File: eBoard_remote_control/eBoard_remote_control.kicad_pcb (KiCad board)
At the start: 2 copper layers, 34 x 99.9 mm, 57 parts, among them J1 SWDIO_conn, J2 105450-0101, U1 MDBT42, U2 AP2112(3.3V), U3 MCP73831T-2ACI/OT, U4 CP2104, U5 AH49ENTR-G1, U6 AH49ENTR-G1, U7 AH49ENTR-G1, U8 SSD1306, X1 JSTPH, X2 JSTPH, X4 32.768

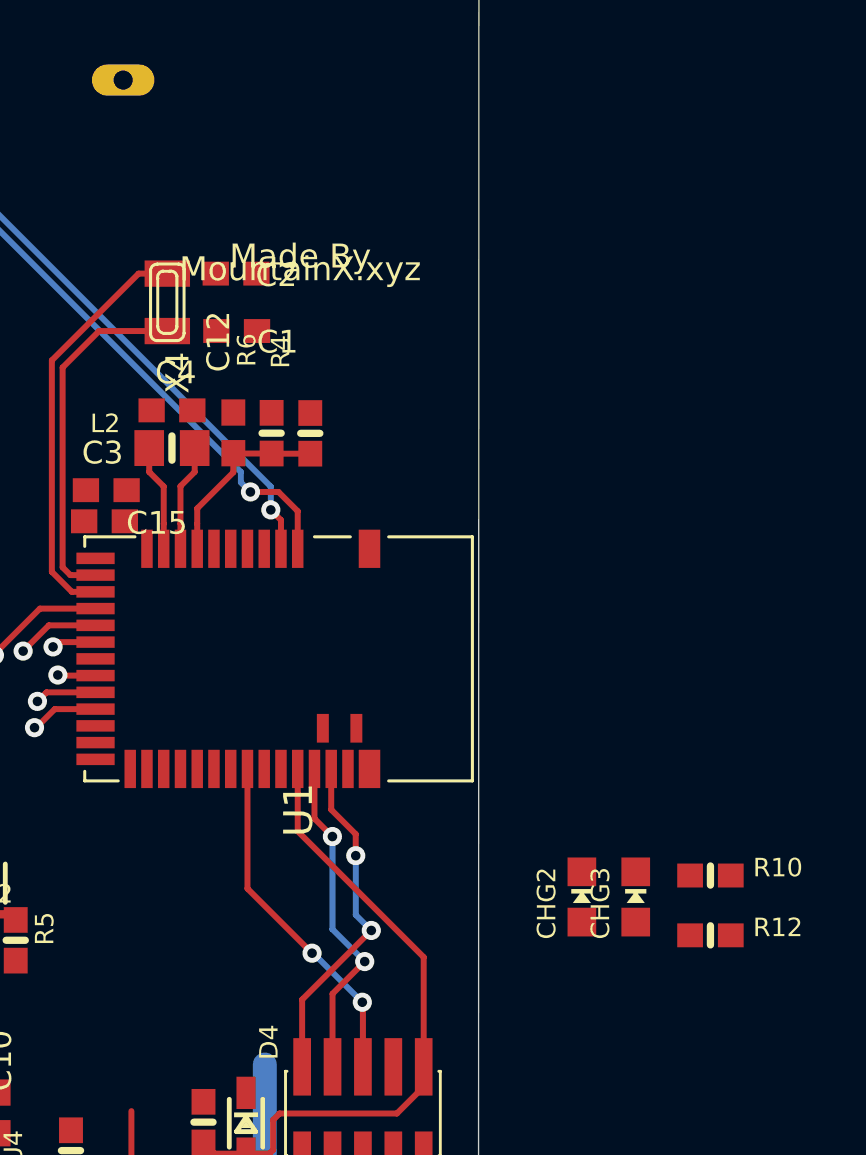
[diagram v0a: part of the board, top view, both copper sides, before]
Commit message: updated 3d modelis
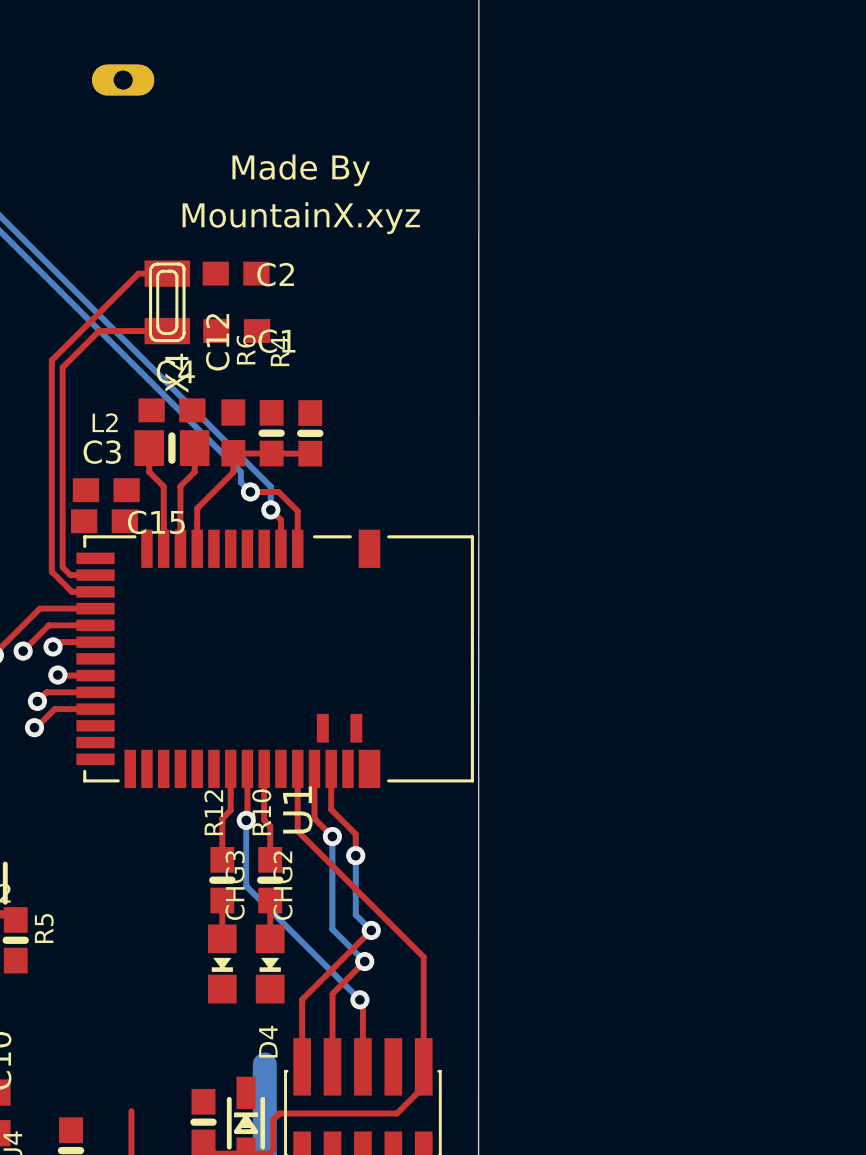
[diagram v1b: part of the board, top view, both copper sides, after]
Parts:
- moved R12 20.5 mm to (200.8, 132.2), turned to 90 degrees
- moved R10 18.4 mm to (202.8, 132.2), turned to 90 degrees
- moved CHG3 17.5 mm to (200.8, 135.8), turned to 180 degrees
- moved CHG2 13.3 mm to (202.8, 135.8), turned to 180 degrees
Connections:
- U1 pad 31: (no net) -> Net-(R12-Pad2)
- U1 pad 33: (no net) -> Net-(R10-Pad2)
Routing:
- net Net-(R12-Pad2): track 0.00 -> 3.94 mm
- net Net-(R10-Pad2): track 0.00 -> 3.90 mm
- net Net-(CHG3-PadA): track 0.00 -> 1.60 mm
- net Net-(CHG2-PadA): track 0.00 -> 1.60 mm
